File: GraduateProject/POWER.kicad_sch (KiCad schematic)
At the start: 24 parts, among them J2 Conn_01x04_Pin, U2 L7815, U3 L7805, U4 L7805, U6 EL357N(D)(TA)-G_C42385002

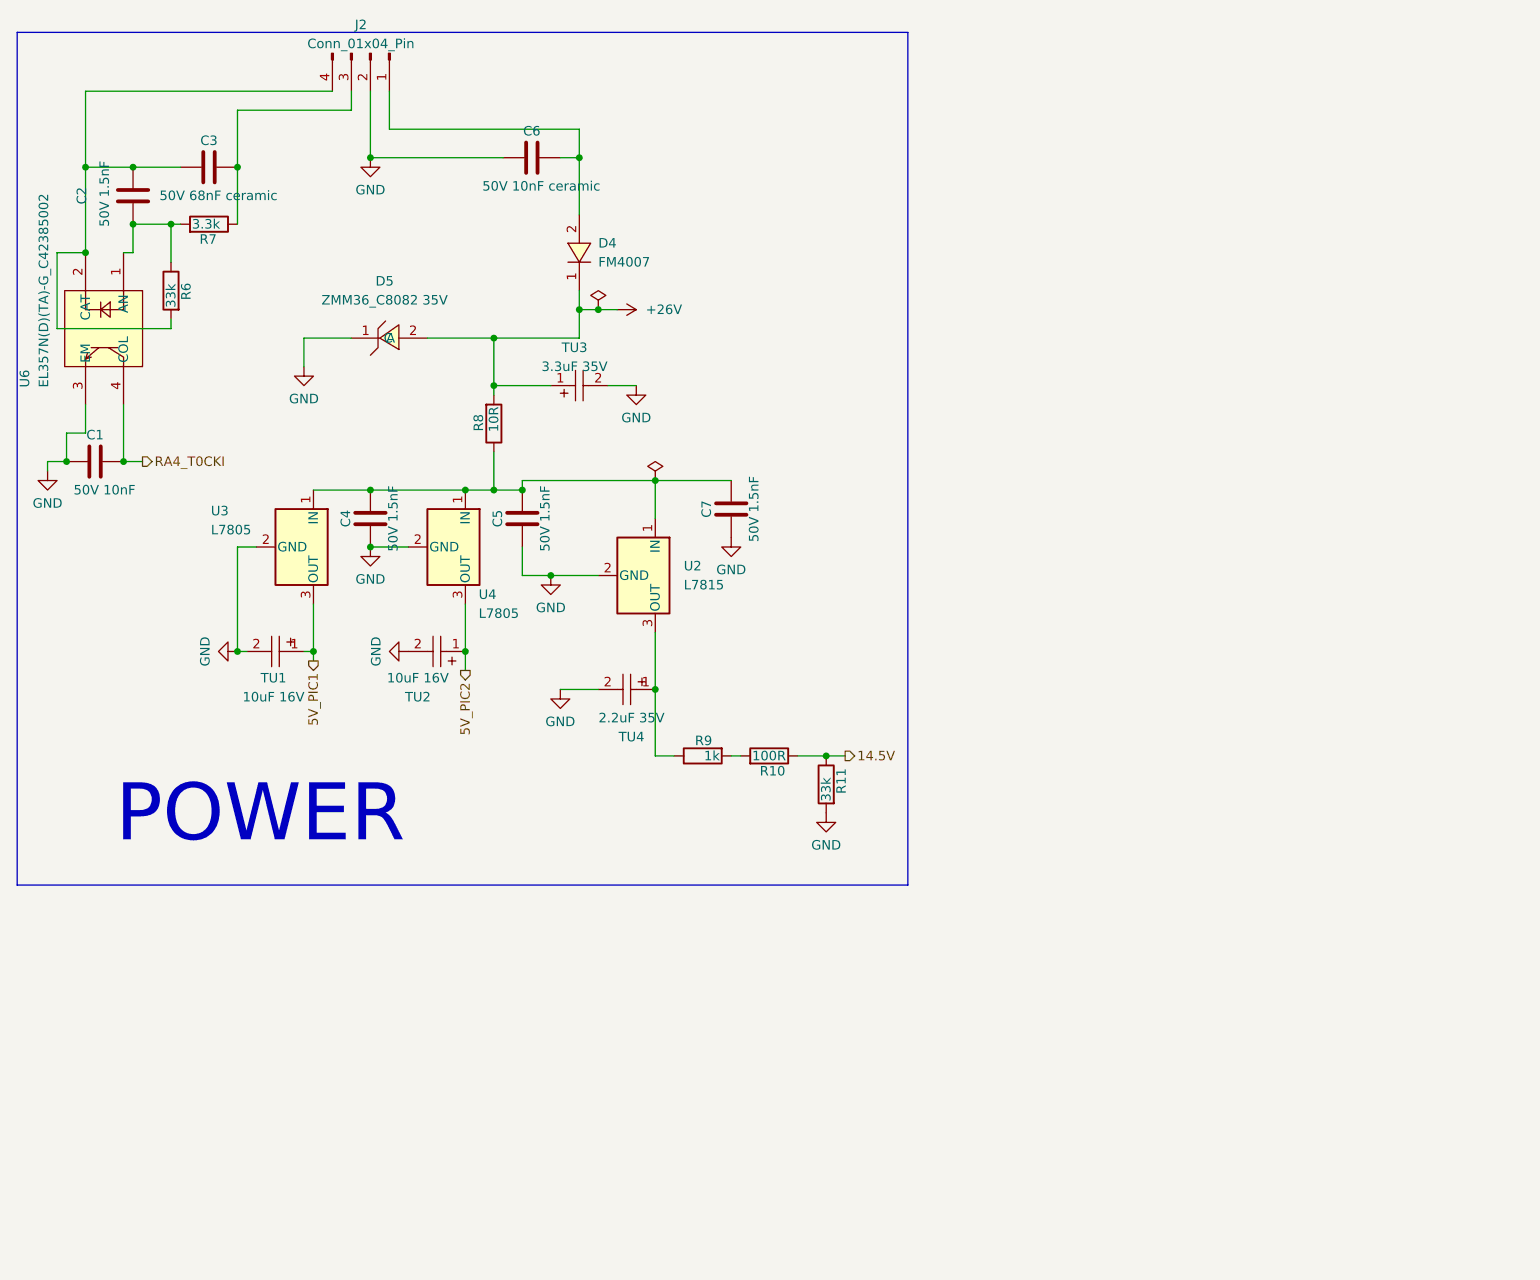
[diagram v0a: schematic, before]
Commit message: Add files via upload
5/10/25
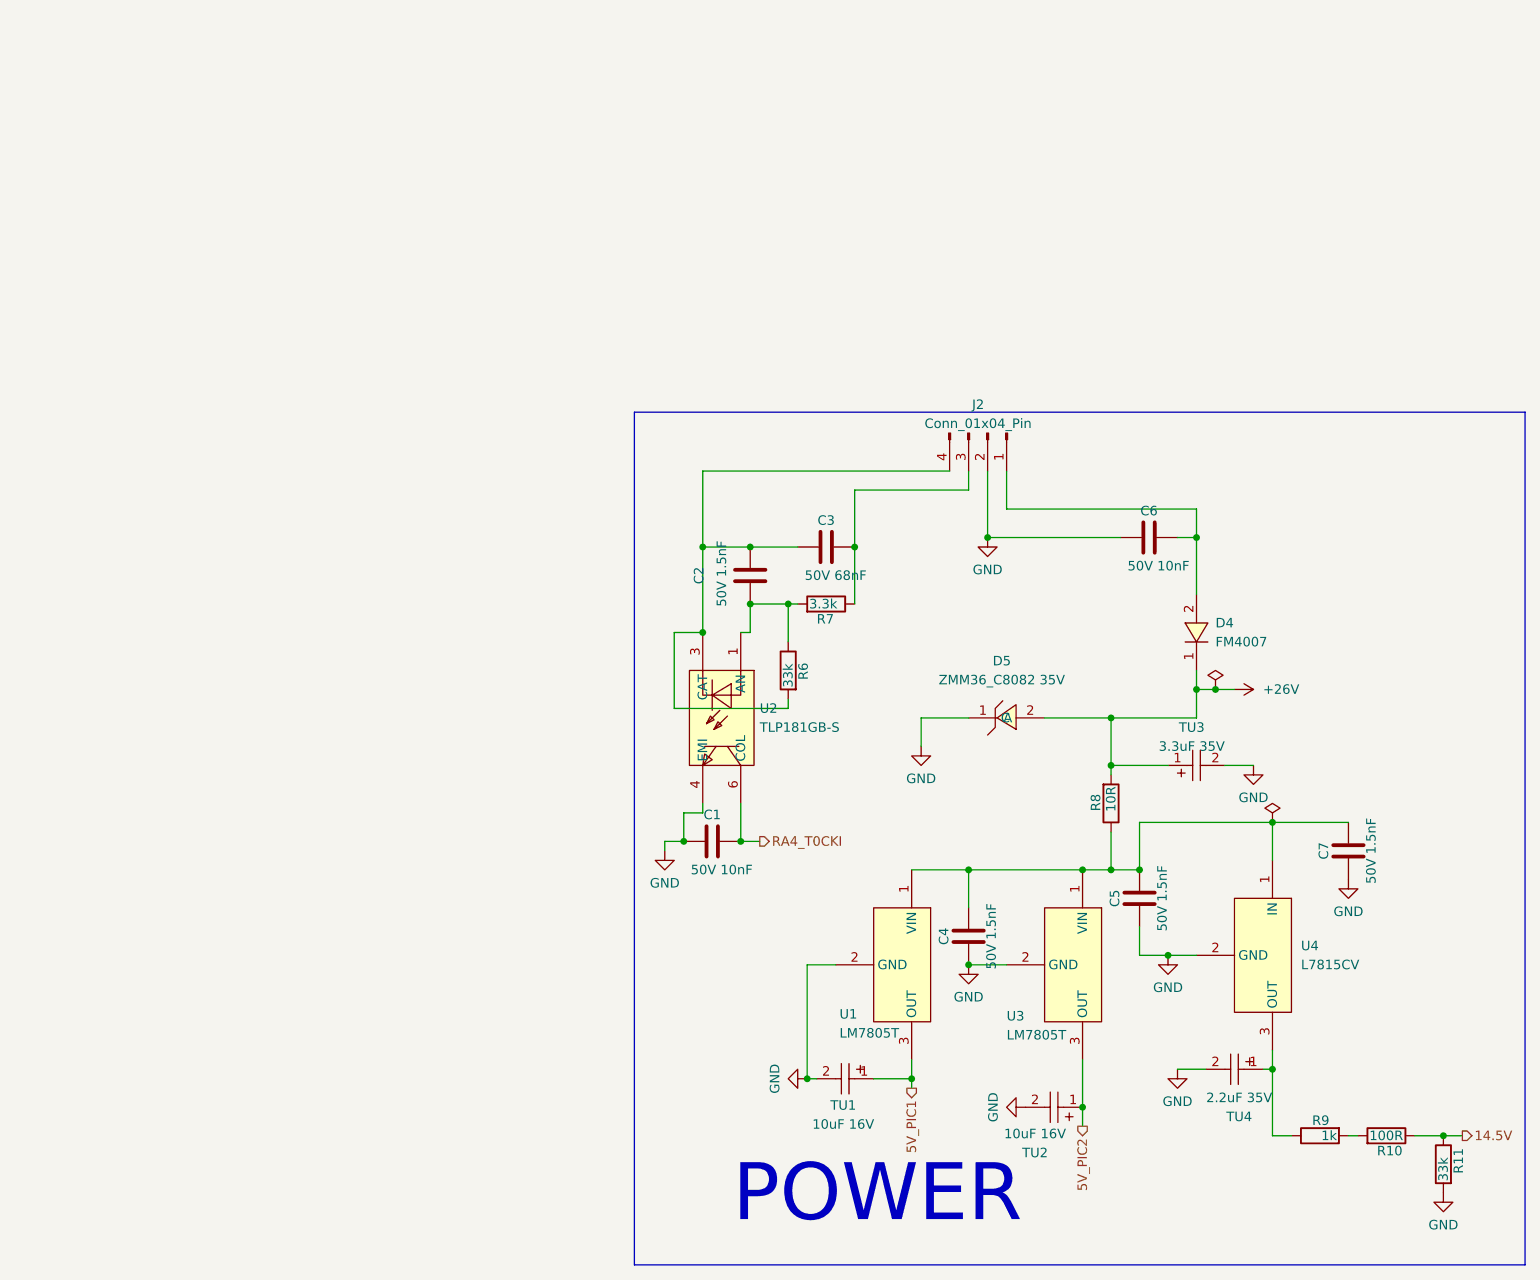
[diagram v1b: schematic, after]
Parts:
- removed U2: L7815, Package_TO_SOT_SMD:TO-263-2, symbol Regulator_Linear:L7815
- removed U3, U4: L7805, Package_TO_SOT_SMD:TO-263-2, symbol Regulator_Linear:L7805
- removed U6: EL357N(D)(TA)-G_C42385002, easyeda2kicad:SOP-4_L3.9-W4.4-P2.54-LS7.0-TL, symbol easyeda2kicad:EL357N(D)(TA)-G_C42385002
- added U1, U3: LM7805T, easyeda2kicad:TO-220-3_L10.0-W4.5-P2.54-L, symbol easyeda2kicad:LM7805T
- added U2: TLP181GB-S, easyeda2kicad:SOP-4_L3.7-W4.6-P2.54-LS7.0-TL, symbol easyeda2kicad:TLP181GB-S
- added U4: L7815CV, easyeda2kicad:TO-220-3_L10.0-W4.5-P2.54-L, symbol easyeda2kicad:L7815CV
- C1: Buying link (none) -> https://www.thegioiic.com/tu-gom-0805-10nf-50v
- C2, C4, C5, C7: Buying link (none) -> https://www.thegioiic.com/tu-gom-0805-1-5nf-50v
- C3: value 50V 68nF ceramic -> 50V 68nF; Buying link (none) -> https://www.thegioiic.com/tu-gom-0805-68nf-50v
- C6: value 50V 10nF ceramic -> 50V 10nF; Buying link (none) -> https://www.thegioiic.com/tu-gom-1206-10nf-50v
- D5: Buying link (none) -> https://www.thegioiic.com/zmm36-diode-zener-36v-500mw-sod-80
- R10: Buying link (none) -> https://www.thegioiic.com/dien-tro-100-ohm-0805-1-
- R11, R6: Buying link (none) -> https://www.thegioiic.com/dien-tro-33-kohm-0805-1-
- R7: Buying link (none) -> https://www.thegioiic.com/dien-tro-3-3-kohm-0805-1-
- R8: Buying link (none) -> https://www.thegioiic.com/dien-tro-10-ohm-0805-1-
- R9: Buying link (none) -> https://www.thegioiic.com/dien-tro-1-kohm-0805-1-
- TU1, TU2: Buying link (none) -> https://www.thegioiic.com/tu-tantalum-10uf-16v-2312-tajc106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
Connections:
- net 5V_PIC1: now also U1.3 (OUT)
- net 5V_PIC2: now also U3.3 (OUT)
- net GND: now also U1.2 (GND), U2.4 (EMI), U3.2 (GND), U4.2 (GND)
- net RA4_T0CKI: now also U2.6 (COL)
- net at C2.2, R6.1, R7.2: now also U2.1 (AN)
- net at C2.1, C3.2, J2.4 (Pin_4)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: now also U2.3 (CAT)
- net at R9.1, TU4.1: now also U4.3 (OUT)
- net at C4.1, C5.1, C7.1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: now also U1.1 (VIN), U3.1 (VIN), U4.1 (IN)
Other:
- moved on the sheet: C1, C2, C3, C4, C5, C6, C7, D4, D5, J2, R10, R11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
